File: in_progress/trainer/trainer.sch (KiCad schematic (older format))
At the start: 18 parts

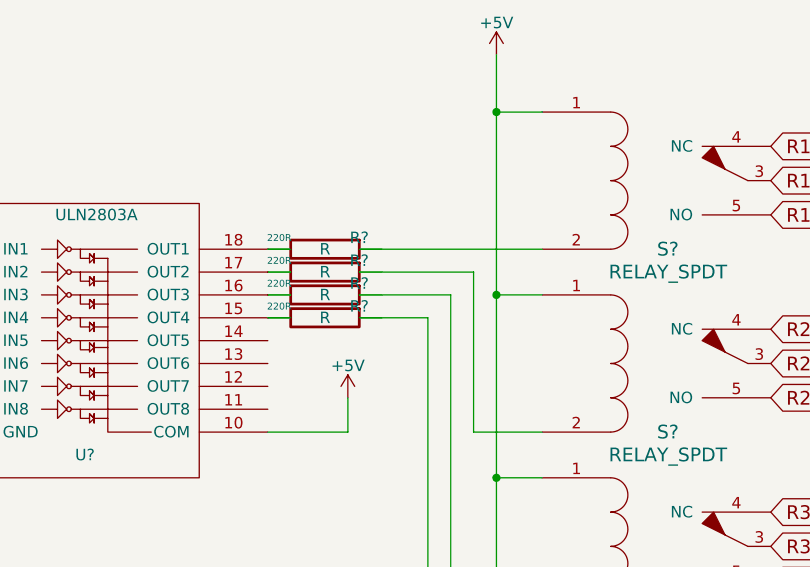
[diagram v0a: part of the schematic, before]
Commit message: .
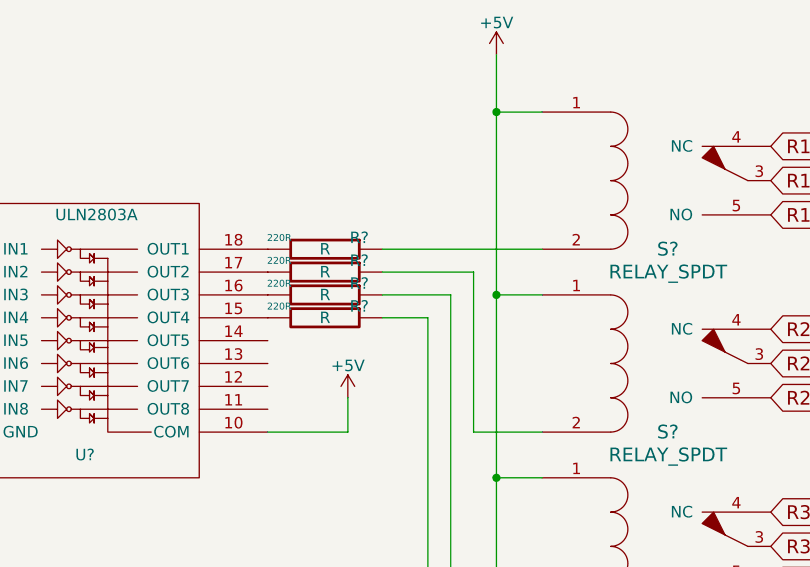
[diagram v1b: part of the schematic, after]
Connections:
- wire segments 44 -> 40
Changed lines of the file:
@@
-EESchema Schematic File Version 2  date 08/12/2015 11:18:57
+EESchema Schematic File Version 2
 LIBS:trainer-rescue
 LIBS:power
@@
 LIBS:valves
 LIBS:MiscellaneousDevices
-LIBS:ULN280xA
 LIBS:Gajda_cmosieee
 LIBS:jhd-162a
 LIBS:capteurs
 LIBS:trainer-cache
-EELAYER 27 0
+EELAYER 25 0
 EELAYER END
 $Descr A4 11693 8268
@@
 	3500 3100 3500 2750
 Wire Wire Line
-	3000 4800 3100 4800
-Wire Wire Line
-	3000 4900 3100 4900
-Wire Wire Line
-	3000 5000 3100 5000
-Wire Wire Line
-	3000 5100 3100 5100
-Wire Wire Line
 	4000 3950 4000 6600
 Wire Wire Line
@@
 Connection ~ 4000 5800
 Wire Wire Line
-	4200 4800 3400 4800
+	4200 4800 3500 4800
 Wire Wire Line
 	4200 5600 3900 5600
@@
 	3900 5600 3900 4900
 Wire Wire Line
-	3900 4900 3400 4900
+	3900 4900 3500 4900
 Wire Wire Line
 	4200 6400 3800 6400
@@
 	3800 6400 3800 5000
 Wire Wire Line
-	3800 5000 3400 5000
+	3800 5000 3500 5000
 Wire Wire Line
 	4200 7200 3700 7200
@@
 	3700 7200 3700 5100
 Wire Wire Line
-	3700 5100 3400 5100
+	3700 5100 3500 5100
 $Comp
 L GNDREF #PWR?

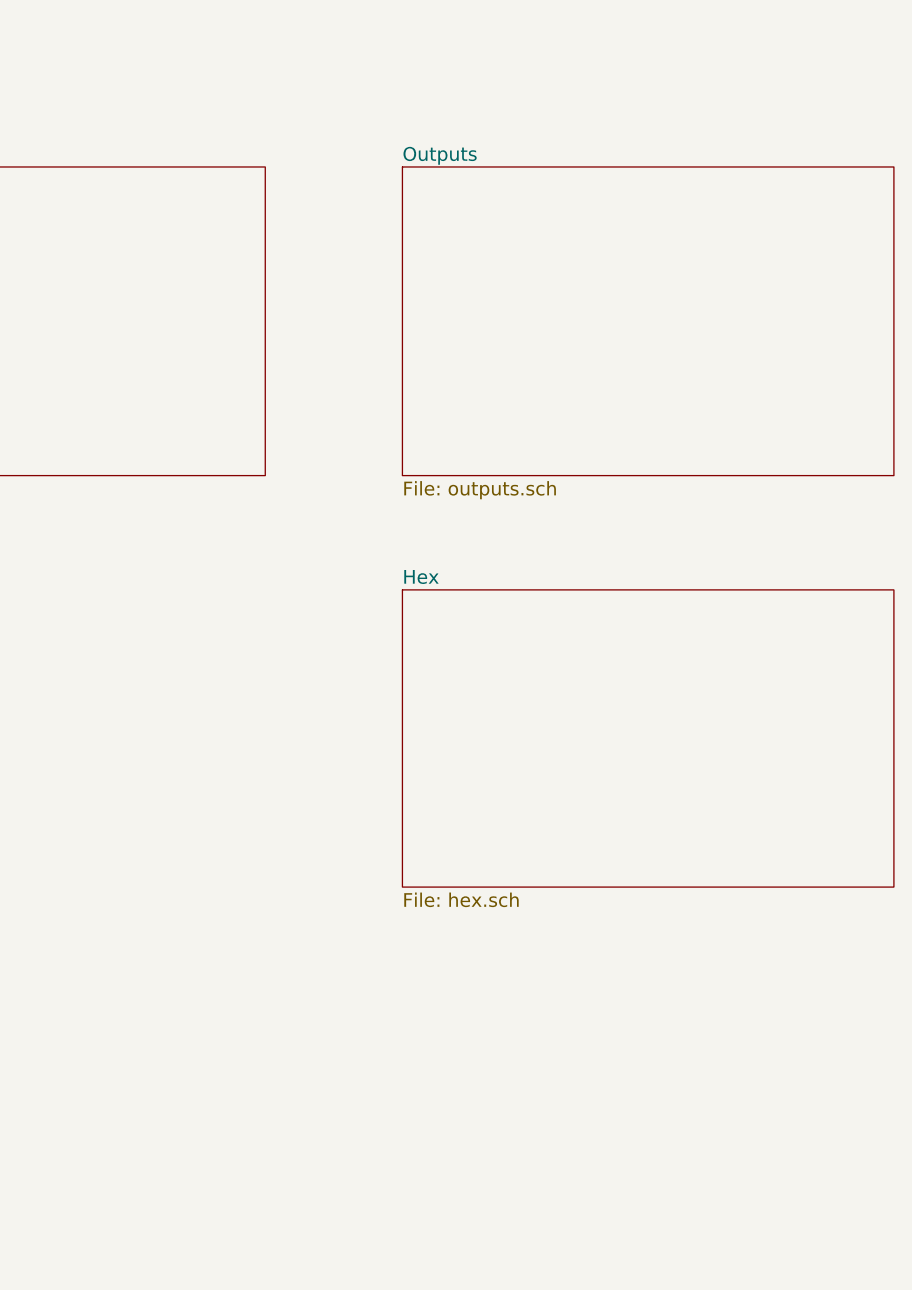
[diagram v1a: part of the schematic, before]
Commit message: .
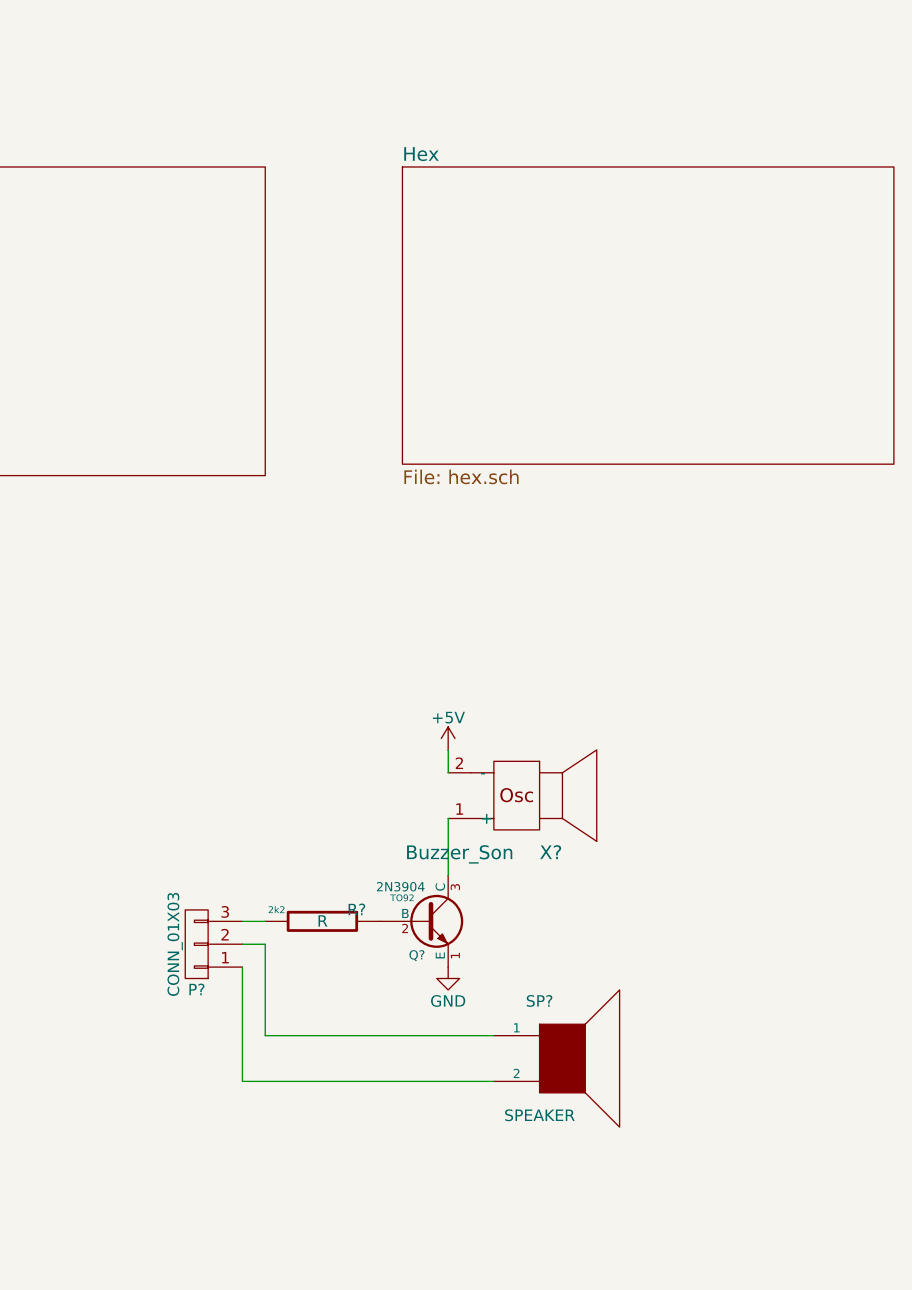
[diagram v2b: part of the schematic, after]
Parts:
- added P?: CONN_01X03, symbol CONN_01X03
- added Q?: 2N3904, TO92, symbol PN2222A-RESCUE-trainer
- added R?: R, 2k2, symbol R-RESCUE-trainer
- added SP?: SPEAKER, symbol SPEAKER
- added X?: Buzzer_Son, symbol Buzzer_Son
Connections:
- net labels added: GND
- wire segments 40 -> 48
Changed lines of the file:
@@
 $Descr A4 11693 8268
 encoding utf-8
-Sheet 1 4
+Sheet 1 3
 Title ""
 Date "8 dec 2015"
@@
 F1 "inputs.sch" 60
 $EndSheet
-$Sheet
-S 8300 1300 2150 1350
-U 56560475
-F0 "Outputs" 60
-F1 "outputs.sch" 60
-$EndSheet
 $Comp
 L RELAY_SPDT S?
@@
 Isolated power supply\n(powers internal LEDs, ICs)
 $Sheet
-S 8300 3150 2150 1300
+S 8300 1300 2150 1300
 U 565EDE3C
 F0 "Hex" 60
 F1 "hex.sch" 60
 $EndSheet
+$Comp
+L CONN_01X03 P?
+U 1 1 5669F9CF
+P 7400 4700
+F 0 "P?" H 7400 4900 50  0000 C CNN
+F 1 "CONN_01X03" V 7500 4700 50  0000 C CNN
+F 2 "" H 7400 4700 60  0000 C CNN
+F 3 "" H 7400 4700 60  0000 C CNN
+	1    7400 4700
+	-1   0    0    1
+$EndComp
+$Comp
+L SPEAKER SP?
+U 1 1 5669F9D6
+P 9000 5200
+F 0 "SP?" H 8900 5450 50  0000 C CNN
+F 1 "SPEAKER" H 8900 4950 50  0000 C CNN
+F 2 "" H 9000 5200 60  0000 C CNN
+F 3 "" H 9000 5200 60  0000 C CNN
+	1    9000 5200
+	1    0    0    -1
+$EndComp
+$Comp
+L Buzzer_Son X?
+U 1 1 5669F9DD
+P 8800 4050
+F 0 "X?" H 8650 4300 60  0000 C CNN
+F 1 "Buzzer_Son" H 9050 4300 60  0000 C CNN
+F 2 "" H 8800 4050 60  0000 C CNN
+F 3 "" H 8800 4050 60  0000 C CNN
+	1    8800 4050
+	-1   0    0    1
+$EndComp
+$Comp
+L +5V #PWR?
+U 1 1 5669F9E4
+P 8500 3850
+F 0 "#PWR?" H 8500 3700 50  0001 C CNN
+F 1 "+5V" H 8500 3990 50  0000 C CNN
+F 2 "" H 8500 3850 60  0000 C CNN
+F 3 "" H 8500 3850 60  0000 C CNN
+	1    8500 3850
+	1    0    0    -1
+$EndComp
+Wire Wire Line
+	7600 4600 7700 4600
+Wire Wire Line
+	7600 4800 7600 5300
+Wire Wire Line
+	7600 5300 8700 5300
+Wire Wire Line
+	7600 4700 7700 4700
+Wire Wire Line
+	7700 4700 7700 5100
+Wire Wire Line
+	7700 5100 8700 5100
+$Comp
+L PN2222A-RESCUE-trainer Q?
+U 1 1 5669F9F0
+P 8400 4600
+F 0 "Q?" H 8400 4452 40  0000 R CNN
+F 1 "2N3904" H 8400 4750 40  0000 R CNN
+F 2 "TO92" H 8300 4702 29  0000 C CNN
+F 3 "~" H 8400 4600 60  0000 C CNN
+	1    8400 4600
+	1    0    0    -1
+$EndComp
+$Comp
+L R-RESCUE-trainer R?
+U 1 1 5669F9F7
+P 7950 4600
+F 0 "R?" V 7900 4750 50  0000 C CNN
+F 1 "R" V 7950 4600 50  0000 C CNN
+F 2 "2k2" V 7900 4400 30  0000 C CNN
+F 3 "" H 7950 4600 30  0000 C CNN
+	1    7950 4600
+	0    1    1    0
+$EndComp
+$Comp
+L GND #PWR?
+U 1 1 5669F9FE
+P 8500 4800
+F 0 "#PWR?" H 8500 4550 50  0001 C CNN
+F 1 "GND" H 8500 4650 50  0000 C CNN
+F 2 "" H 8500 4800 50  0000 C CNN
+F 3 "" H 8500 4800 50  0000 C CNN
+	1    8500 4800
+	1    0    0    -1
+$EndComp
+Wire Wire Line
+	8500 4150 8500 4400
+Wire Wire Line
+	8500 3950 8500 3850
 $EndSCHEMATC

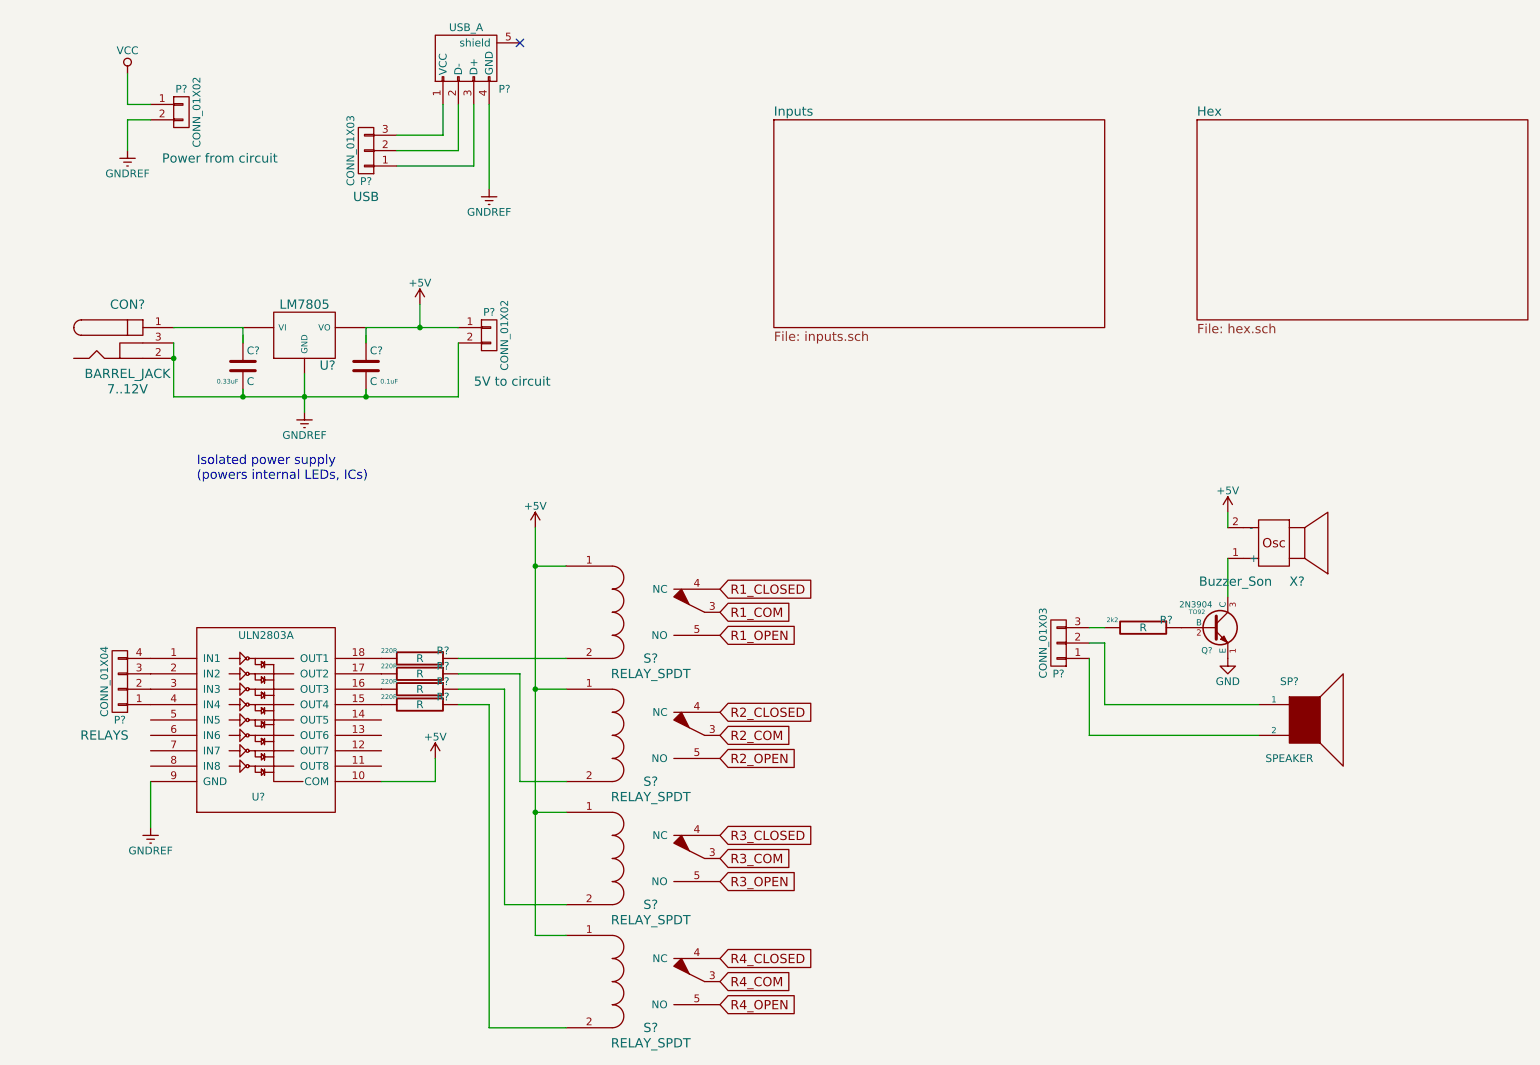
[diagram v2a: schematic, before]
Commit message: .
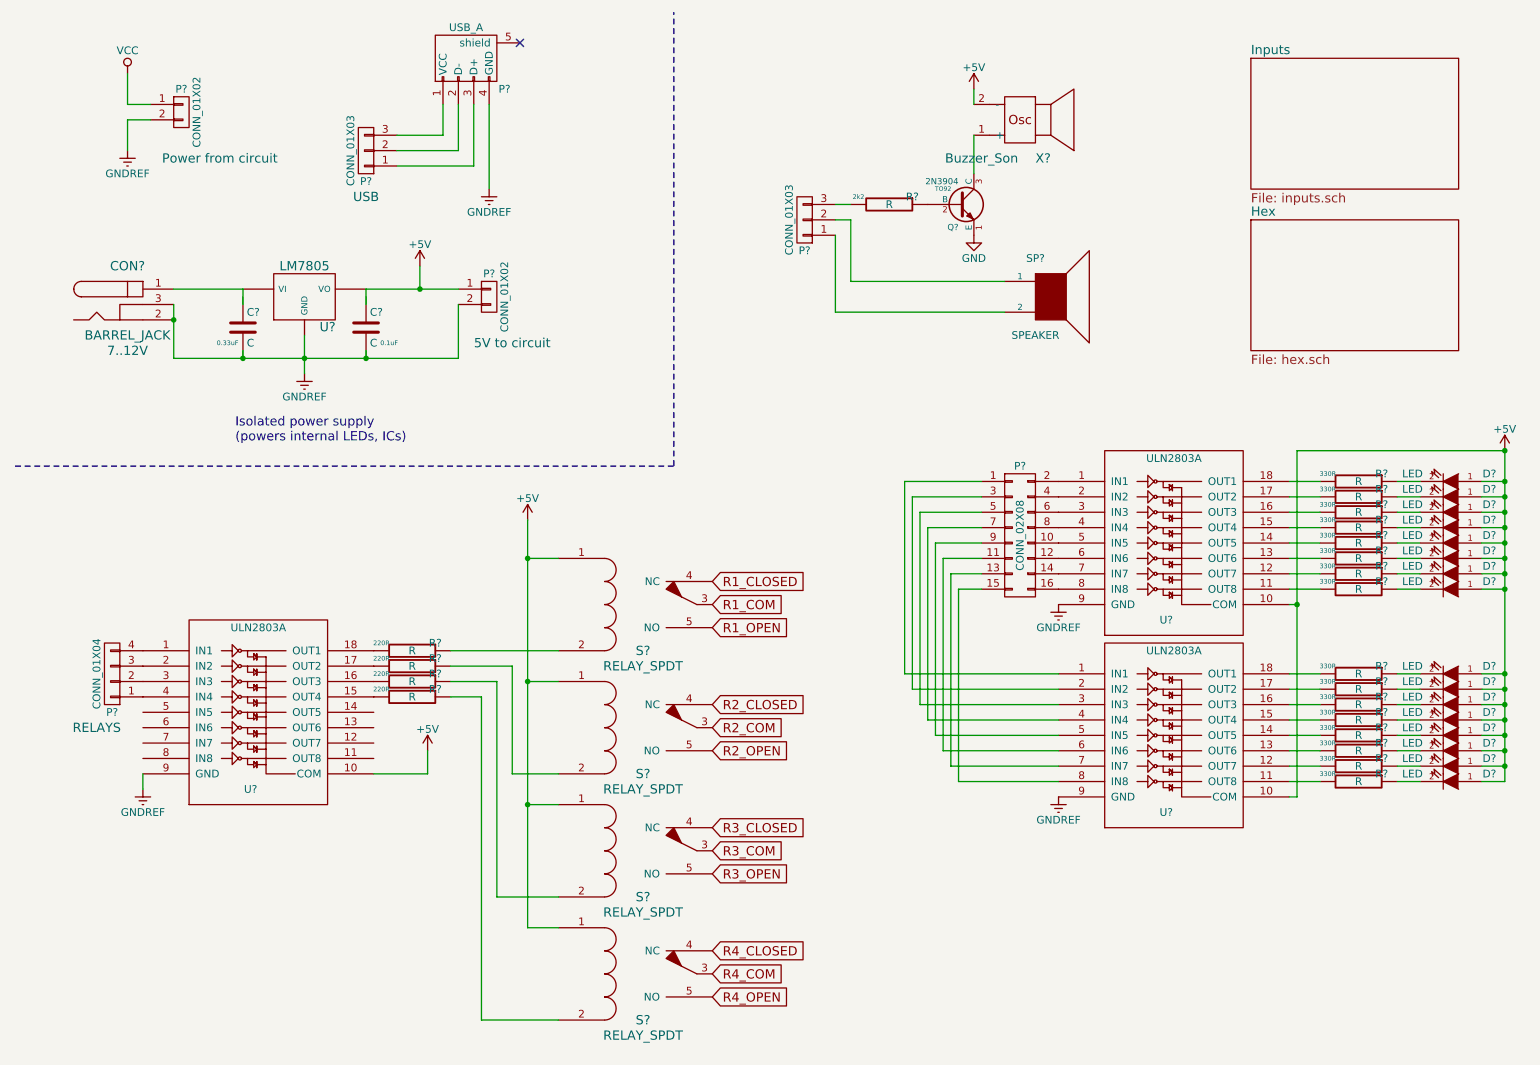
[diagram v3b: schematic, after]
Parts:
- added D? (x16): LED, symbol LED-RESCUE-trainer
- added P?: CONN_02X08, symbol CONN_02X08
- added R? (x16): R, 330R, symbol R-RESCUE-trainer
- added U? (x2): ULN2803A, symbol ULN2803A
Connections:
- wire segments 48 -> 125
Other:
- moved on the sheet: C?, CON?, P?, Q?, R?, S?, SP?, U?, X?

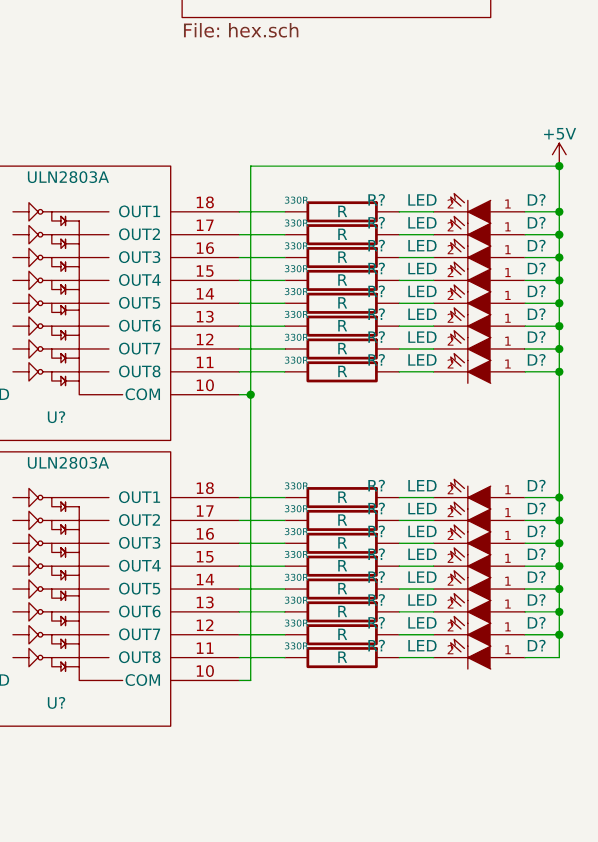
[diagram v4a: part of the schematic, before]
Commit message: .
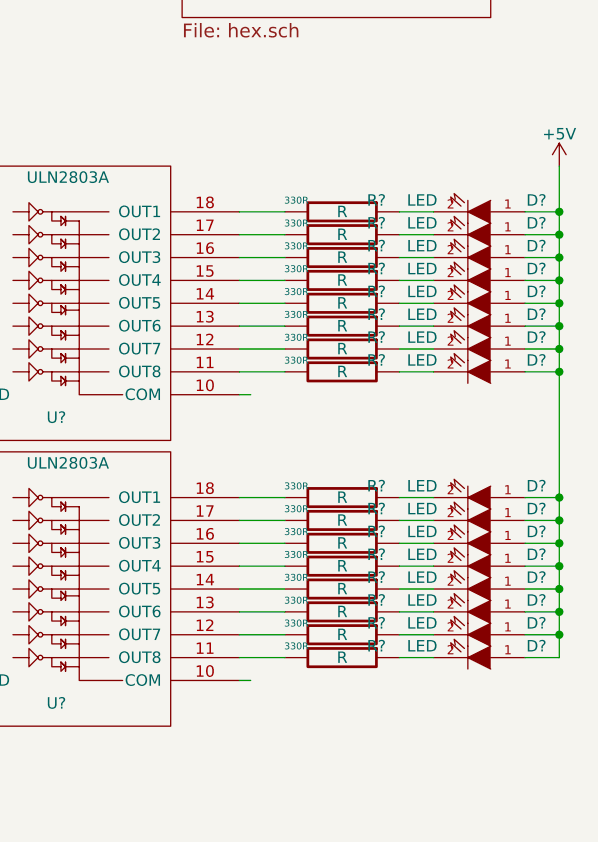
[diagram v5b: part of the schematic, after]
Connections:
- wire segments 125 -> 123
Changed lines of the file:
@@
 Wire Wire Line
 	8950 5700 8900 5700
-Connection ~ 8950 4450
 Wire Wire Line
 	10300 3650 10150 3650
-Wire Wire Line
-	8950 3450 10300 3450
 Wire Wire Line
 	10300 3450 10300 5600
@@
 Connection ~ 10300 5500
 Wire Wire Line
-	8950 3450 8950 5700
-Connection ~ 10300 3450
-Wire Wire Line
 	9600 4350 9750 4350
